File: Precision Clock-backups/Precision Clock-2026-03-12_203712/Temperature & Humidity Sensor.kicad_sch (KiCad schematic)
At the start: 8 parts, among them Q3 DMN3008SFG

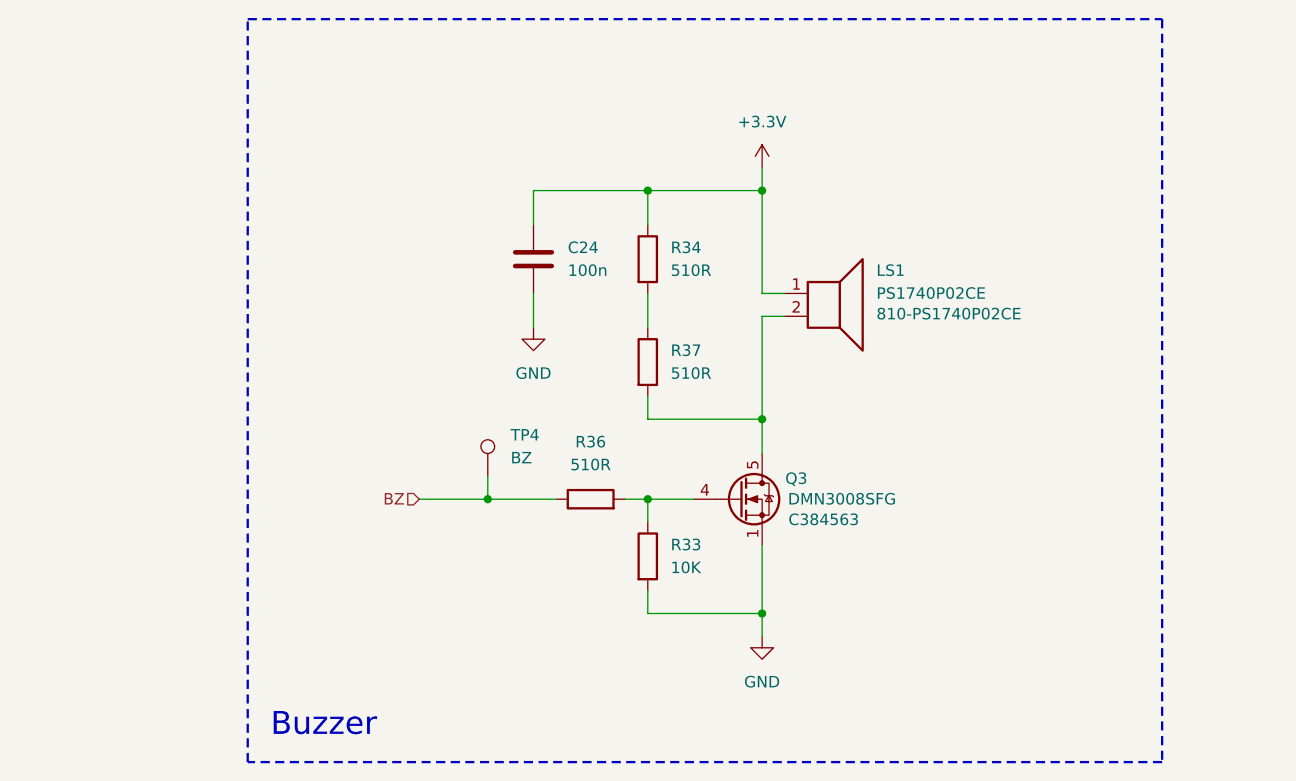
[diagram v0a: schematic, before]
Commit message: Routing
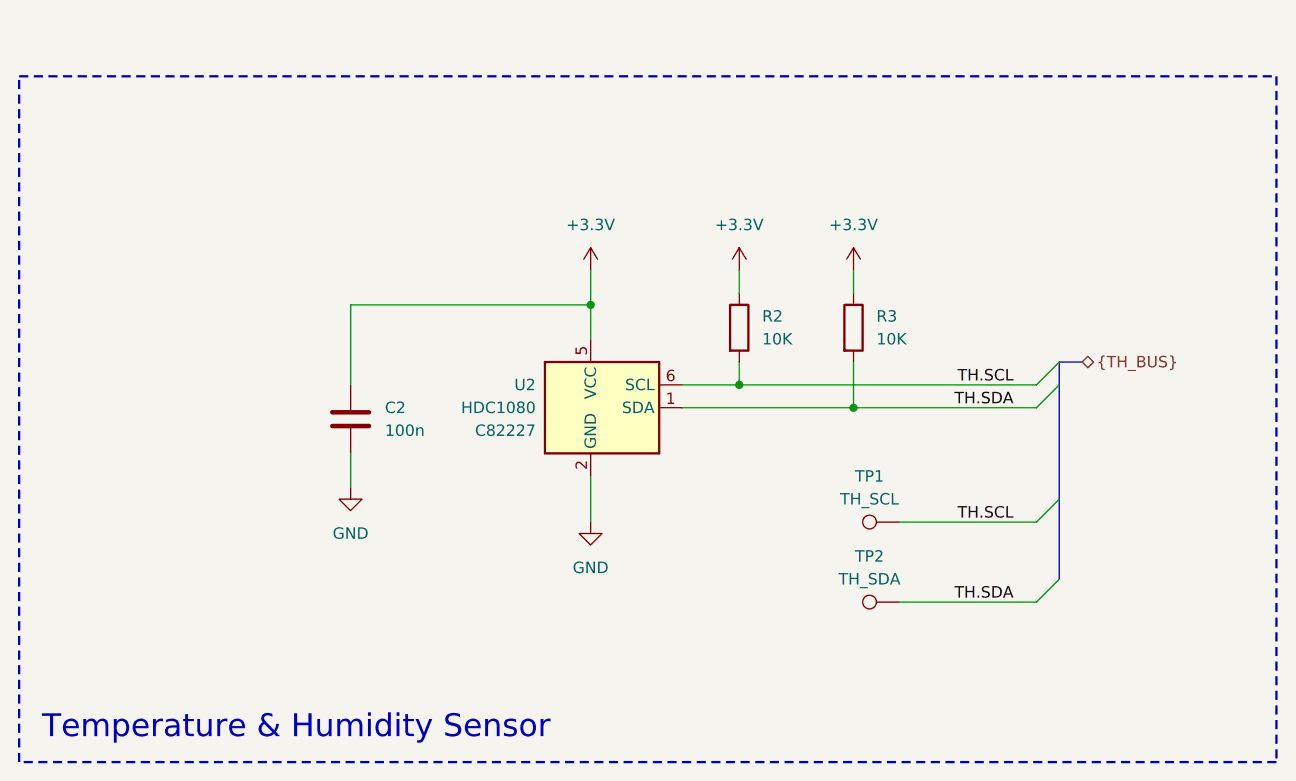
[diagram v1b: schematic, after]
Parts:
- removed C24: 100n, Capacitor_SMD:C_0402_1005Metric, symbol Device:C
- removed LS1: PS1740P02CE, precision_clock:TDK PS1740P02CE, symbol Device:Speaker
- removed Q3: DMN3008SFG, Package_SON:Diodes_PowerDI3333-8, symbol Transistor_FET:DMN3008SFG
- removed R33: 10K, Resistor_SMD:R_0402_1005Metric, symbol Device:R
- removed R34, R36, R37: 510R, Resistor_SMD:R_0402_1005Metric, symbol Device:R
- removed TP4: BZ, TestPoint:TestPoint_Pad_D1.0mm, symbol Connector:TestPoint
- added C2: 100n, Capacitor_SMD:C_0402_1005Metric, symbol Device:C
- added R2, R3: 10K, Resistor_SMD:R_0402_1005Metric, symbol Device:R
- added TP1: TH_SCL, TestPoint:TestPoint_Pad_D1.0mm, symbol Connector:TestPoint
- added TP2: TH_SDA, TestPoint:TestPoint_Pad_D1.0mm, symbol Connector:TestPoint
- added U2: HDC1080, Package_SON:Texas_PWSON-N6, symbol Sensor_Humidity:HDC1080
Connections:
- net +3.3V: now also C2.1, R2.1, R3.1, U2.5 (VCC)
- net GND: now also C2.2, U2.2 (GND)
- new net TH.SCL: R2.2, TP1.1, U2.6 (SCL)
- new net TH.SDA: R3.2, TP2.1, U2.1 (SDA)
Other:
- note added: "Temperature & Humidity Sensor"
- note removed: "Buzzer"
- title: Buzzer -> Temperature & HumiditySensor
